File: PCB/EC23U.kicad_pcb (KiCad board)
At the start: 2 copper layers, 77.2 x 137.6 mm, 79 parts, among them J1 JST, J2 RGB, SW1 BOOT0, SW10 EC_SW, SW11 EC_SW, SW12 EC_SW, SW13 EC_SW, SW14 EC_SW, SW15 EC_SW, SW16 EC_SW, SW17 EC_SW, SW18 EC_SW, SW19 EC_SW, SW2 EC_SW, SW20 EC_SW, SW21 EC_SW, SW22 EC_SW, SW23 EC_SW, SW24 EC_SW, SW25 EC_SW, SW26 EC_SW, SW27 EC_SW, SW28 EC_SW, SW3 EC_SW, SW4 EC_SW, SW5 EC_SW, SW6 EC_SW, SW7 EC_SW, SW8 EC_SW, SW9 EC_SW, U1 STM32F401CBUx, U2 XC6206PxxxMR, U3 74HC4051, U4 OPA350, U5 SN74AHCT1G125, Y1 8 MHz

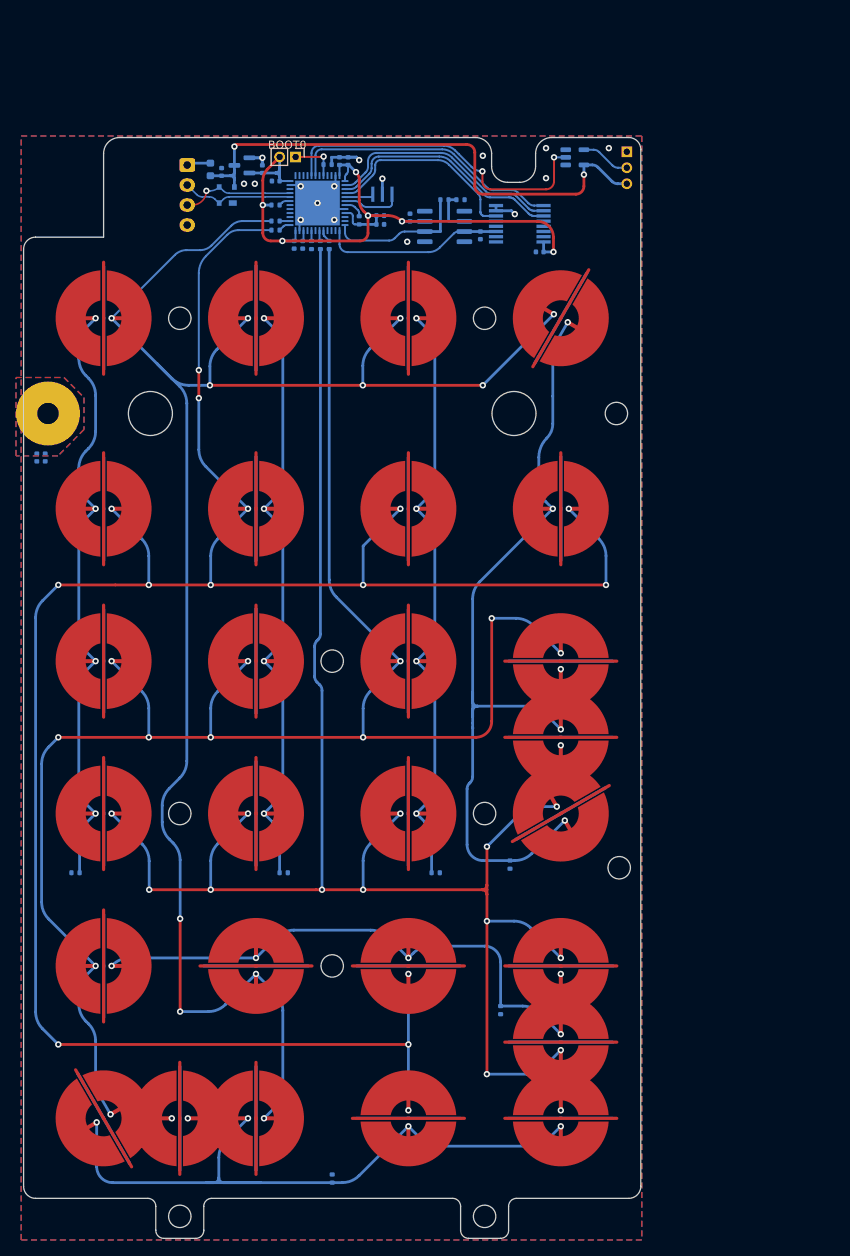
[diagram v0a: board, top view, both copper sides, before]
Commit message: WIP PCB
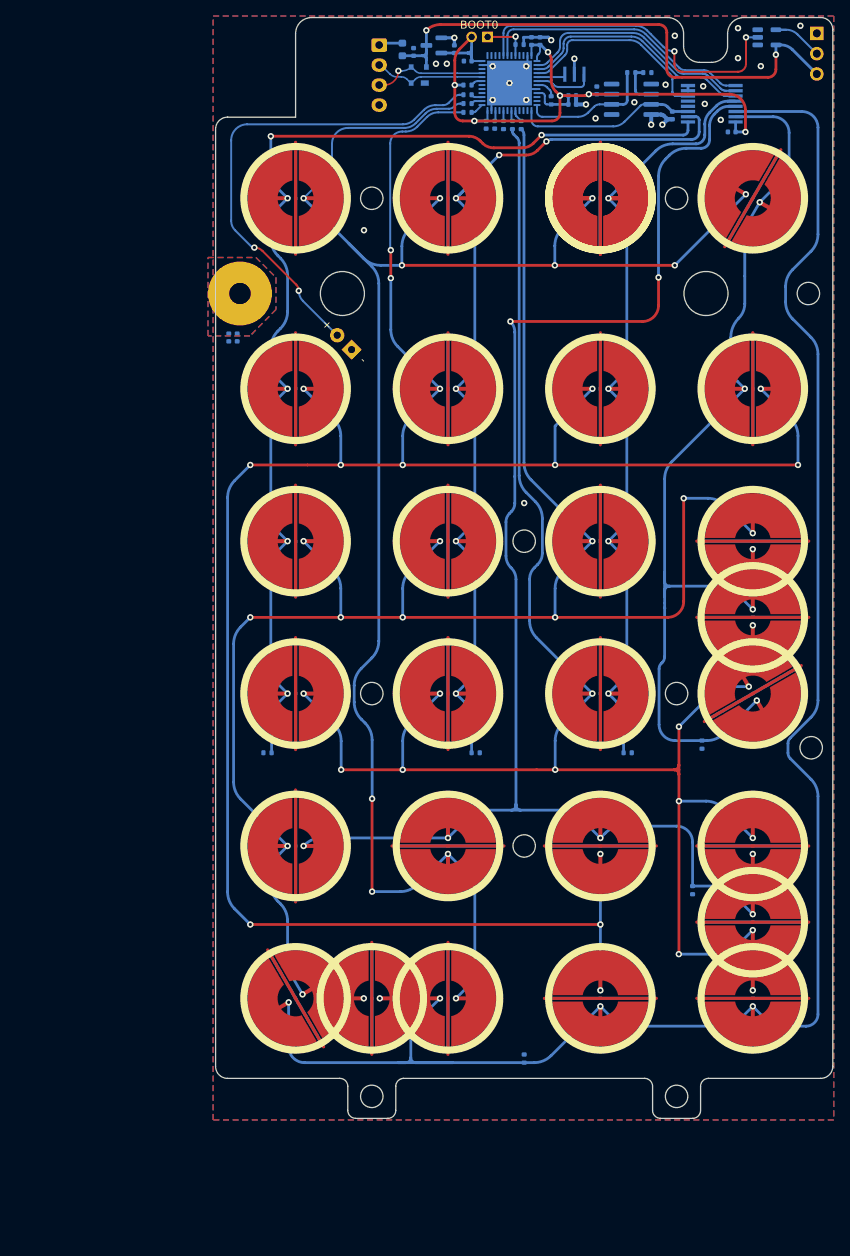
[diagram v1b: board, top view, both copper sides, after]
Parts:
- added D2: LED, LED_THT:LED_D3.0mm, F.Cu at (106.1, 67.9)
- added G***: LOGO, LOGO, B.Cu at (161.4, 157.0)
- added G***: LOGO, LOGO, B.Cu at (126.8, 60.9)
- added G***: LOGO, cipulot_parts:Cipulot_all_info, B.Cu at (152.5, 82.6)
- added R18: 100, Resistor_SMD:R_0402_1005Metric, B.Cu at (120.6, 36.1)
- added SW4: EC_SW, cipulot_parts:ecs_pad_no_ring, F.Cu at (137.2, 49.0)
- J2: footprint Connector_PinSocket_2.00mm:PinSocket_1x03_P2.00mm_Vertical -> Connector_PinSocket_2.54mm:PinSocket_1x03_P2.54mm_Vertical
- moved R9 57.7 mm to (148.7, 135.5), turned to -90 degrees
- moved R14 52.2 mm to (121.6, 118.3), turned to 0 degrees
- moved H11 28.3 mm to (146.7, 161.3)
- moved H2 28.3 mm to (146.7, 49.0)
- moved H6 28.3 mm to (146.7, 110.9)
- moved H9 28.3 mm to (163.2, 60.9)
- moved SW5 28.3 mm to (156.2, 49.0)
- moved C1 28.3 mm to (124.0, 39.8)
- moved C13 28.3 mm to (90.7, 66.4)
- moved C2 28.3 mm to (113.8, 30.7)
- moved C3 28.3 mm to (118.9, 30.4)
- moved C5 28.3 mm to (122.9, 39.8)
- moved C7 28.3 mm to (128.6, 29.4)
- moved C8 28.3 mm to (133.7, 36.2)
- moved C9 28.3 mm to (133.7, 37.3)
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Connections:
- R10 pad 1: SENSE_4 -> SENSE_5
- R13 pad 1: SENSE_1 -> SENSE_0
- R14 pad 1: SENSE_0 -> SENSE_1
- R9 pad 1: SENSE_5 -> SENSE_4
- U1 pad 27: unconnected-(U1-Pad27) -> Num_Lock_Led
- U3 pad 1: SENSE_1 -> SENSE_0
- U3 pad 13: SENSE_5 -> SENSE_4
- U3 pad 14: SENSE_4 -> SENSE_5
- U3 pad 2: SENSE_0 -> SENSE_1
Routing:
- net SENSE_5: track 85.6 -> 223.1 mm
- net SENSE_4: track 67.3 -> 181.5 mm, vias 5 -> 7
- net SENSE_0: track 75.5 -> 138.5 mm, vias 4 -> 6
- net Net-(D2-Pad2): track 0.00 -> 61.4 mm, vias 0 -> 2
- net SENSE_1: track 75.0 -> 115.2 mm, vias 4 -> 6
- net SENSE_2: track 74.8 -> 96.8 mm
- net SENSE_3: track 101.5 -> 119.3 mm
- net GND: track 20.2 -> 25.6 mm, vias 16 -> 26
- net STROBE_3: track 219.0 -> 213.8 mm, vias 15 -> 14
- net STROBE_0: track 222.8 -> 224.7 mm
- net Num_Lock_Led: track 0.00 -> 1.40 mm
- net LED_5V: track 6.20 -> 7.45 mm
- net ADC: track 17.7 -> 16.7 mm
- net VBAT: track 90.4 -> 91.1 mm
- net +5V: track 67.7 -> 68.4 mm
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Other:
- board size 77.2 x 137.6 mm -> 77.1 x 137.6 mm
- board text added: "+"
- board text added: "-"
